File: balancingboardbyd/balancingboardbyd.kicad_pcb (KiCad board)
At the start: 2 copper layers, 52.5 x 189.3 mm, 81 parts, among them CN1 XT30PW-M, CN2 WJ15EDGRC-3.81-4P, CN3 WJ15EDGRC-3.81-4P, Q1 KMBTA94, Q10 SI2302A-TP, Q11 IRFH5302TRPBF, Q2 SI2302A-TP, Q3 SI2302A-TP, Q4 SI2302A-TP, Q5 SI2302A-TP, Q6 KMBTA94, Q7 IRFH5302TRPBF, Q8 NCE0103Y, Q9 SI2302A-TP, U1 BM3451UNDC-T28A, U2 BM3451UNDC-T28A, U3 XT30PW-F, U4 BH-21700-B1BJ001, U5 BH-21700-B1BJ001, U6 BH-21700-B1BJ001, U7 BH-21700-B1BJ001, U8 BH-21700-B1BJ001, U9 BH-21700-B1BJ001

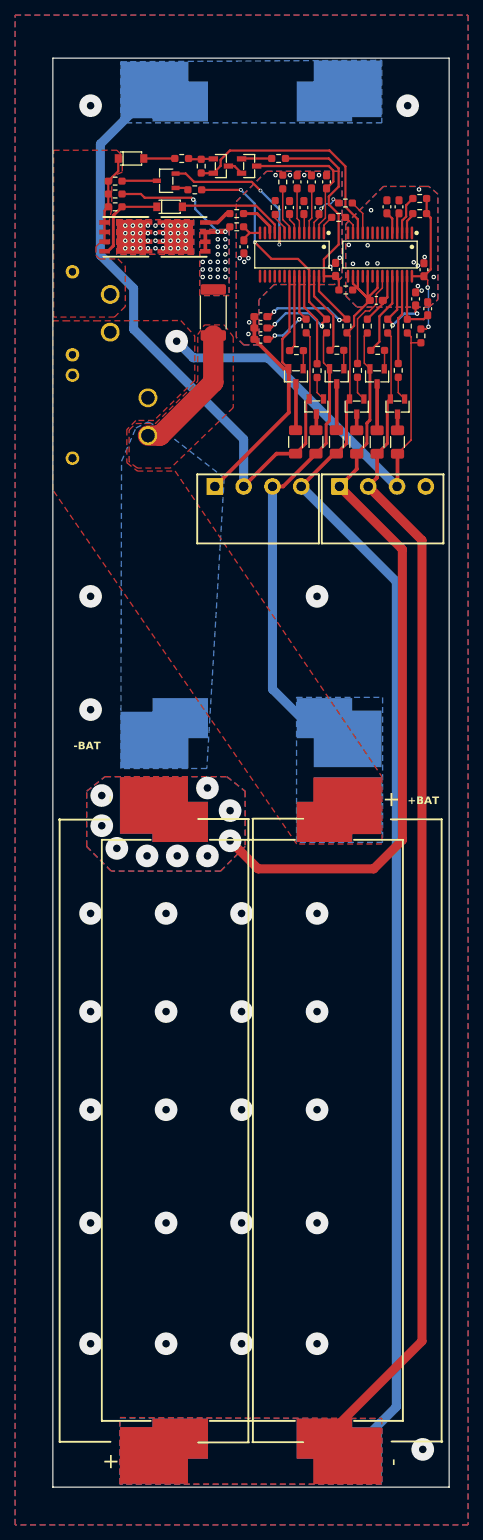
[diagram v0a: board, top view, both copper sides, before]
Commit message: bestelle teile
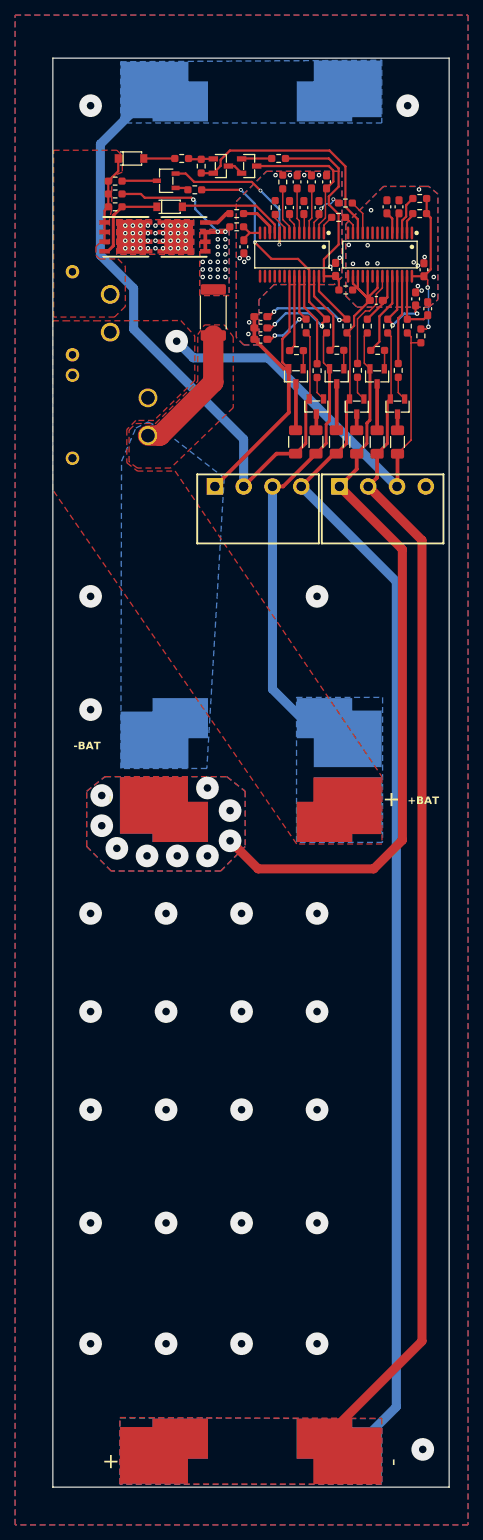
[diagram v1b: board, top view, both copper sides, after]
